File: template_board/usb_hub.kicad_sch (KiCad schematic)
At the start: 11 parts, among them U12 CH334P, Y6 12Mhz

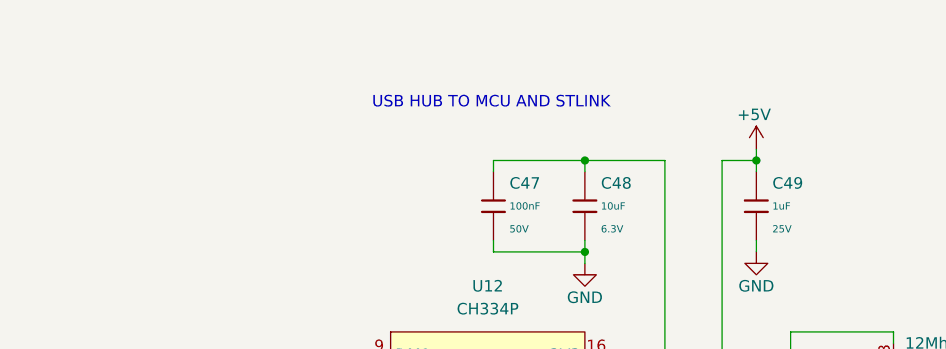
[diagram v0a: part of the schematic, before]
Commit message: chamt skończony chyba
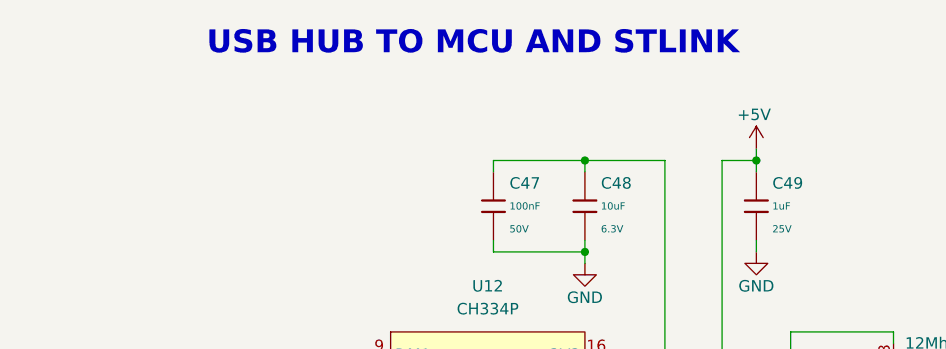
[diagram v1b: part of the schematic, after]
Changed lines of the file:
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@@
 	(text "USB HUB TO MCU AND STLINK"
 		(exclude_from_sim no)
-		(at 153.416 55.88 0)
+		(at 151.384 49.276 0)
 		(effects
 			(font
-				(size 1.27 1.27)
+				(size 2.54 2.54)
+				(thickness 0.508)
+				(bold yes)
 			)
 		)
